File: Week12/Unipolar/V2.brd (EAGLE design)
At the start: 34.8 x 37.8 mm, 13 parts, among them IC1 ATTINY44-SSU

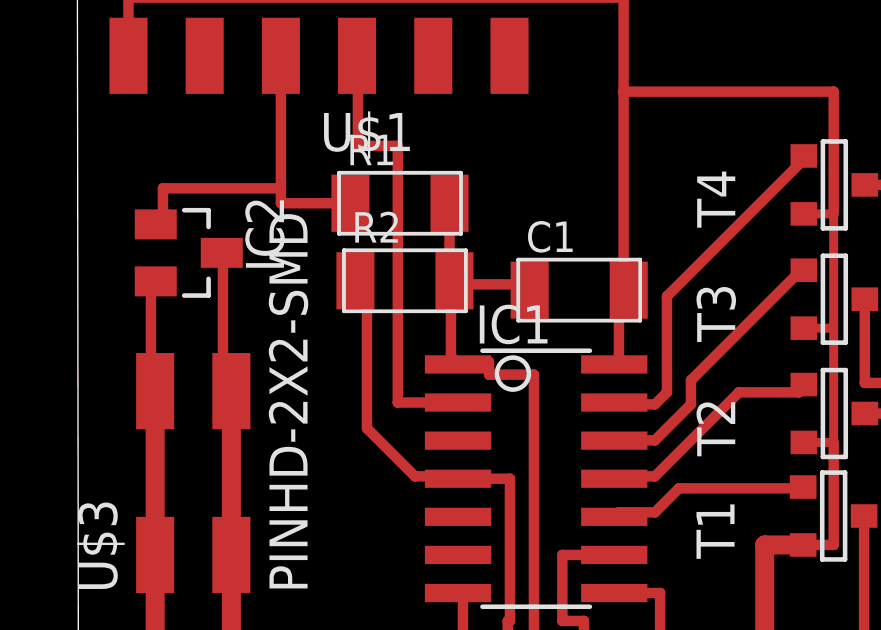
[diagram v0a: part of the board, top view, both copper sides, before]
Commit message: GCodes
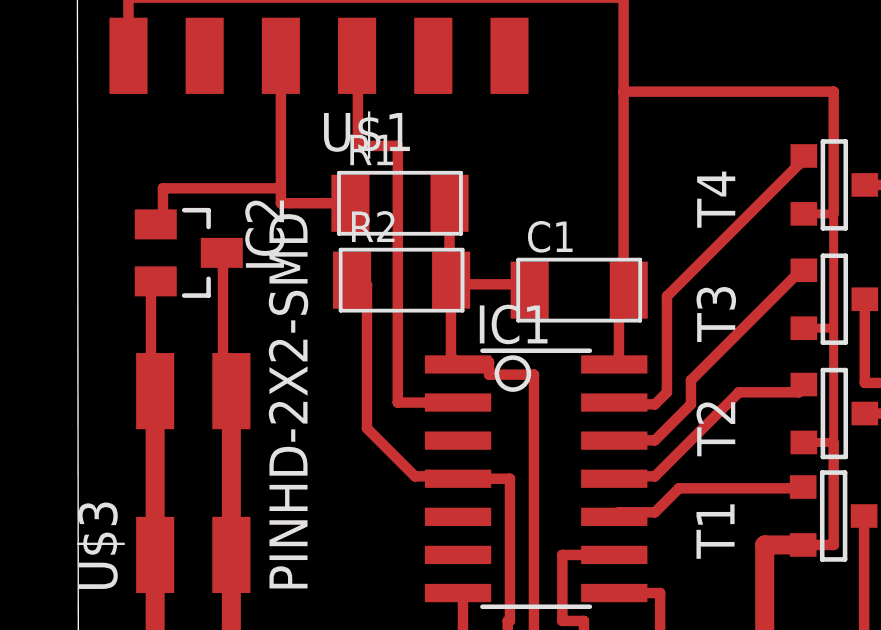
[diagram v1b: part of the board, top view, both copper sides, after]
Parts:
- moved R2 0.11 mm to (10.8, 26.9)
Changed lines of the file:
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@@
 <setting verticaltext="up"/>
 </settings>
-<grid distance="0.1" unitdist="mil" unit="mm" style="lines" multiple="1" display="no" altdistance="5" altunitdist="mil" altunit="mil"/>
+<grid distance="0.1" unitdist="mil" unit="mil" style="lines" multiple="1" display="no" altdistance="5" altunitdist="mil" altunit="mil"/>
 <layers>
-<layer number="1" name="Top" color="4" fill="1" visible="no" active="yes"/>
+<layer number="1" name="Top" color="4" fill="1" visible="yes" active="yes"/>
 <layer number="2" name="Route2" color="16" fill="1" visible="no" active="no"/>
 <layer number="3" name="Route3" color="17" fill="1" visible="no" active="no"/>
@@
 <layer number="17" name="Pads" color="2" fill="1" visible="yes" active="yes"/>
 <layer number="18" name="Vias" color="2" fill="1" visible="yes" active="yes"/>
-<layer number="19" name="Unrouted" color="6" fill="1" visible="no" active="yes"/>
+<layer number="19" name="Unrouted" color="6" fill="1" visible="yes" active="yes"/>
 <layer number="20" name="Dimension" color="24" fill="1" visible="yes" active="yes"/>
-<layer number="21" name="tPlace" color="7" fill="1" visible="no" active="yes"/>
+<layer number="21" name="tPlace" color="7" fill="1" visible="yes" active="yes"/>
 <layer number="22" name="bPlace" color="7" fill="1" visible="yes" active="yes"/>
-<layer number="23" name="tOrigins" color="15" fill="1" visible="no" active="yes"/>
+<layer number="23" name="tOrigins" color="15" fill="1" visible="yes" active="yes"/>
 <layer number="24" name="bOrigins" color="15" fill="1" visible="yes" active="yes"/>
-<layer number="25" name="tNames" color="7" fill="1" visible="no" active="yes"/>
+<layer number="25" name="tNames" color="7" fill="1" visible="yes" active="yes"/>
 <layer number="26" name="bNames" color="7" fill="1" visible="yes" active="yes"/>
-<layer number="27" name="tValues" color="7" fill="1" visible="no" active="yes"/>
+<layer number="27" name="tValues" color="7" fill="1" visible="yes" active="yes"/>
 <layer number="28" name="bValues" color="7" fill="1" visible="yes" active="yes"/>
-<layer number="29" name="tStop" color="7" fill="3" visible="no" active="yes"/>
+<layer number="29" name="tStop" color="7" fill="3" visible="yes" active="yes"/>
 <layer number="30" name="bStop" color="7" fill="6" visible="no" active="yes"/>
-<layer number="31" name="tCream" color="7" fill="4" visible="no" active="yes"/>
+<layer number="31" name="tCream" color="7" fill="4" visible="yes" active="yes"/>
 <layer number="32" name="bCream" color="7" fill="5" visible="no" active="yes"/>
 <layer number="33" name="tFinish" color="6" fill="3" visible="no" active="yes"/>
@@
 <layer number="49" name="Reference" color="7" fill="1" visible="yes" active="yes"/>
 <layer number="50" name="dxf" color="7" fill="1" visible="no" active="no"/>
-<layer number="51" name="tDocu" color="7" fill="1" visible="no" active="yes"/>
+<layer number="51" name="tDocu" color="7" fill="1" visible="yes" active="yes"/>
 <layer number="52" name="bDocu" color="7" fill="1" visible="yes" active="yes"/>
 <layer number="53" name="tGND_GNDA" color="7" fill="9" visible="no" active="no"/>
@@
 <attribute name="VALUE" x="35.3339375" y="6.57098125" size="1.27" layer="27" rot="R90"/>
 </element>
-<element name="R2" library="fab" package="R1206FAB" value="10K" x="10.86611875" y="26.91891875" smashed="yes">
-<attribute name="NAME" x="9.08811875" y="28.18891875" size="1.016" layer="25" ratio="15"/>
-<attribute name="VALUE" x="9.08811875" y="24.63291875" size="1.016" layer="27" ratio="15"/>
+<element name="R2" library="fab" package="R1206FAB" value="10K" x="10.754359375" y="26.9392375" smashed="yes">
+<attribute name="NAME" x="8.976359375" y="28.2092375" size="1.016" layer="25" ratio="15"/>
+<attribute name="VALUE" x="8.976359375" y="24.6532375" size="1.016" layer="27" ratio="15"/>
 </element>
 <element name="T1" library="fab" package="SOT-23" value="" x="25.1561625" y="19.052540625" smashed="yes" rot="R90">
@@
 <wire x1="13.67028125" y1="24.208740625" x2="12.6365" y2="24.208740625" width="0.35" layer="1"/>
 <wire x1="12.6365" y1="24.208740625" x2="12.6365" y2="24.13" width="0.35" layer="1"/>
-<wire x1="12.8" y1="26.8" x2="14.8" y2="26.8" width="0.35" layer="1"/>
+<wire x1="12.736575" y1="26.8" x2="14.8" y2="26.8" width="0.35" layer="1"/>
 <wire x1="14.8" y1="26.8" x2="15.0241" y2="26.6065" width="0.35" layer="1"/>
-<wire x1="12.8" y1="26.8" x2="12.51711875" y2="26.91891875" width="0.35" layer="1"/>
-<wire x1="12.4" y1="24.4" x2="12.4" y2="26.8" width="0.35" layer="1"/>
-<wire x1="12.4" y1="26.8" x2="12.51711875" y2="26.91891875" width="0.35" layer="1"/>
+<wire x1="12.736575" y1="26.8" x2="12.405359375" y2="26.9392375" width="0.35" layer="1"/>
+<wire x1="12.4" y1="24.4" x2="12.4" y2="26.933796875" width="0.35" layer="1"/>
+<wire x1="12.4" y1="26.933796875" x2="12.405359375" y2="26.9392375" width="0.35" layer="1"/>
 <wire x1="12.4" y1="24.4" x2="12.6365" y2="24.13" width="0.35" layer="1"/>
 <wire x1="2.8" y1="28.8" x2="2.8" y2="30" width="0.35" layer="1"/>
@@
 <wire x1="2.8" y1="28.8" x2="2.560134375" y2="28.7985625" width="0.35" layer="1"/>
 <wire x1="6.4" y1="34.4" x2="6.731" y2="34.417" width="0.35" layer="1"/>
-<wire x1="12.4" y1="27.2" x2="12.51711875" y2="26.91891875" width="0.35" layer="1"/>
+<wire x1="12.288240625" y1="27.22031875" x2="12.405359375" y2="26.9392375" width="0.35" layer="1"/>
 <wire x1="2.8" y1="30" x2="6.731" y2="30" width="0.35" layer="1"/>
 <wire x1="6.731" y1="30" x2="6.731" y2="34.417" width="0.35" layer="1"/>
@@
 <wire x1="6.731" y1="29.5021" x2="6.731" y2="30" width="0.35" layer="1"/>
 <wire x1="12.35201875" y1="29.5021" x2="12.35201875" y2="26.8" width="0.35" layer="1"/>
-<wire x1="12.35201875" y1="26.8" x2="12.8" y2="26.8" width="0.35" layer="1"/>
+<wire x1="12.35201875" y1="26.8" x2="12.736575" y2="26.8" width="0.35" layer="1"/>
 <wire x1="12.35201875" y1="29.5021" x2="9.05001875" y2="29.5021" width="0" layer="19" extent="1-1"/>
 </signal>
@@
 <wire x1="14.3664" y1="15.5802" x2="14.3664" y2="20.32" width="0.35" layer="1"/>
 <wire x1="14.3664" y1="20.32" x2="12.6365" y2="20.32" width="0.35" layer="1"/>
-<wire x1="9.6" y1="22" x2="9.6" y2="26.8" width="0.35" layer="1"/>
+<wire x1="9.6" y1="22" x2="9.6" y2="26.7857875" width="0.35" layer="1"/>
 <wire x1="11.2" y1="20.4" x2="9.6" y2="22" width="0.35" layer="1"/>
 <wire x1="12.4" y1="20.4" x2="11.2" y2="20.4" width="0.35" layer="1"/>
-<wire x1="9.6" y1="26.8" x2="9.21511875" y2="26.91891875" width="0.35" layer="1"/>
+<wire x1="9.6" y1="26.7857875" x2="9.103359375" y2="26.9392375" width="0.35" layer="1"/>
 <wire x1="12.4" y1="20.4" x2="12.6365" y2="20.32" width="0.35" layer="1"/>
 </signal>
